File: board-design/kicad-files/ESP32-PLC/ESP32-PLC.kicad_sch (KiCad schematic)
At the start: 41 parts, among them J1 640456-3, J2 Conn_ARM_JTAG_SWD_10, J3 302-S101, J4 302-S101, Q1 BC817, Q2 BC817, U1 BD48ExxG, U2 ESP32-WROVER-E

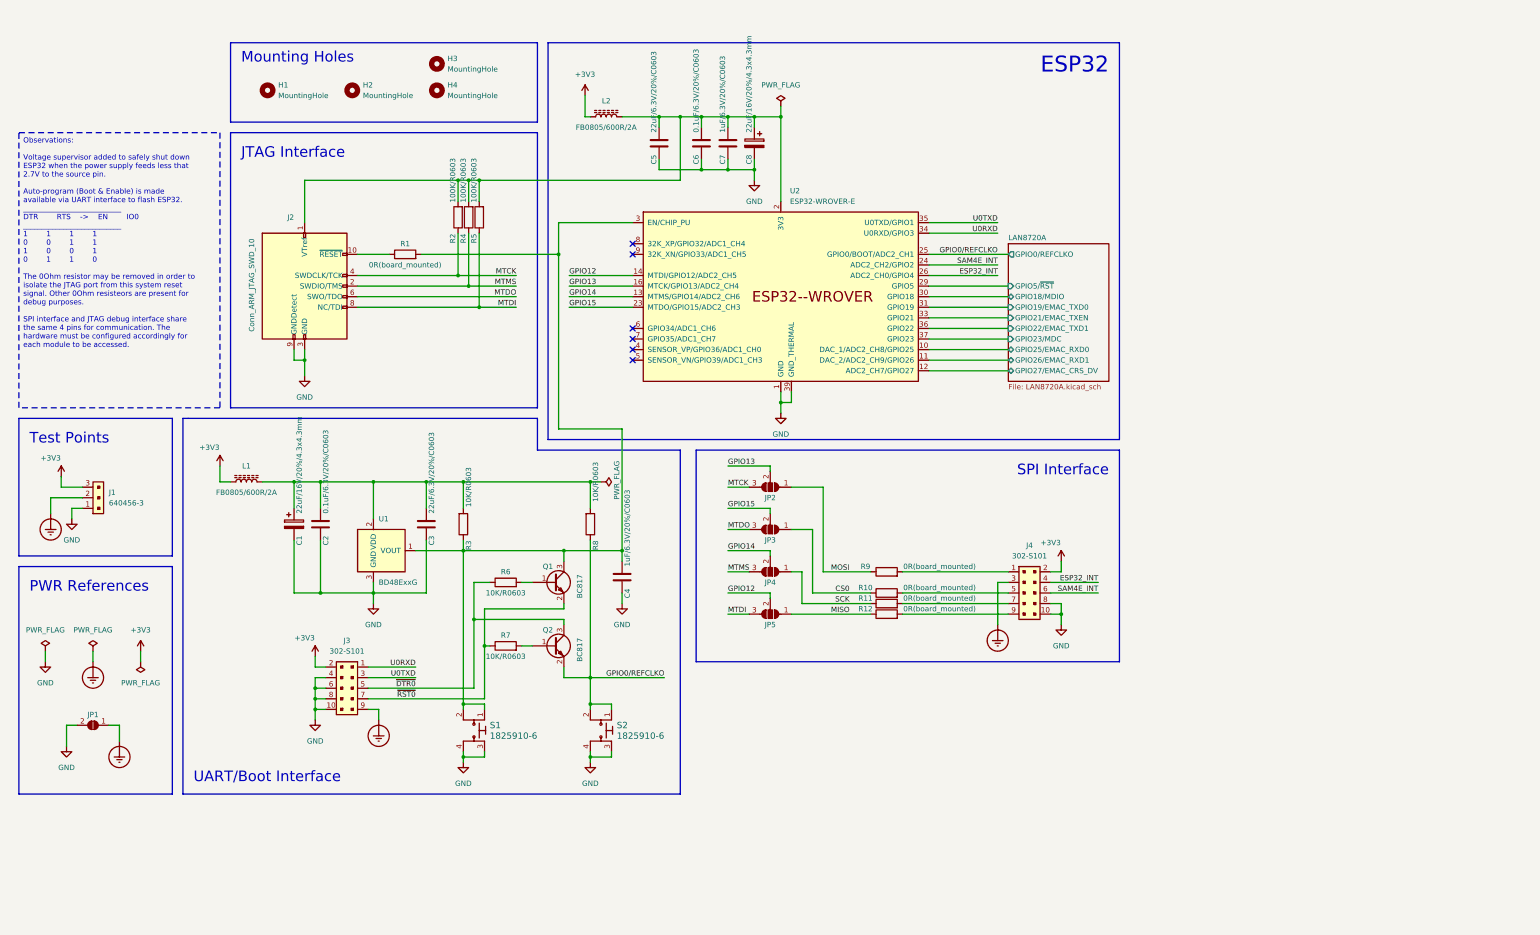
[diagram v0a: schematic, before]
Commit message: [UPDATE]
Work in progress.

Signed-off-by: Nicolae-Andrei Vasile <vasilenicolaeandrei@gmail.com>
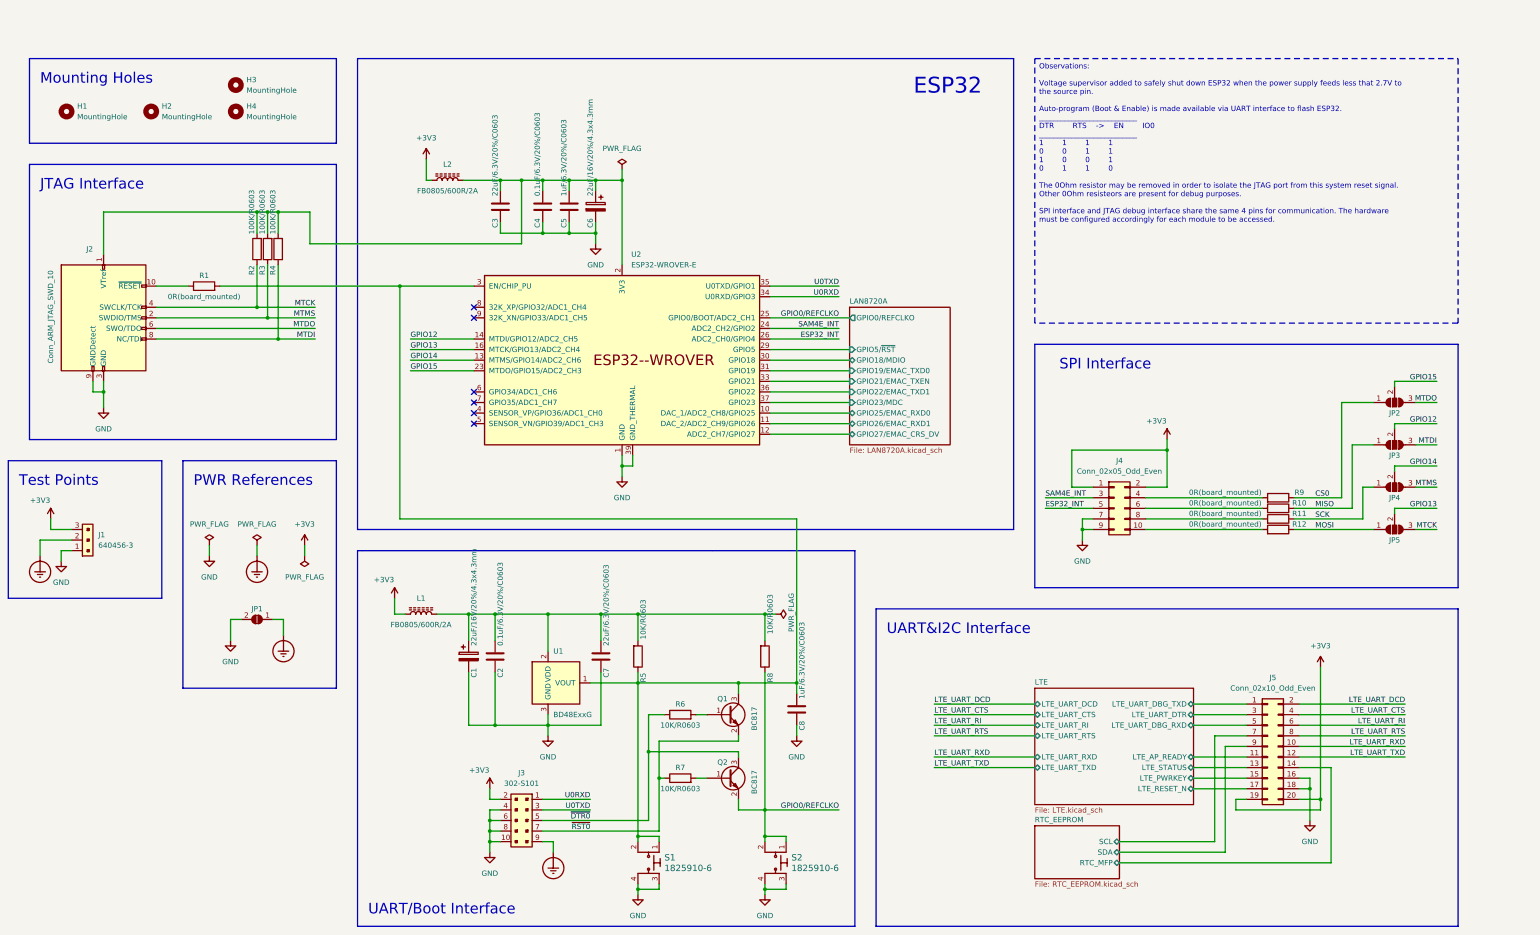
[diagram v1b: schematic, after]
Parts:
- removed J4: 302-S101, Connector_IDC:IDC-Header_2x05_P2.54mm_Vertical, symbol dk_Rectangular-Connectors-Headers-Male-Pins:302-S101
- added J4: Conn_02x05_Odd_Even, Connector_IDC:IDC-Header_2x05_P2.54mm_Vertical, symbol Connector_Generic:Conn_02x05_Odd_Even
- added J5: Conn_02x10_Odd_Even, Connector_IDC:IDC-Header_2x10_P2.54mm_Vertical, symbol Connector_Generic:Conn_02x10_Odd_Even
- renumbered C5 to C3, C6 to C4, C7 to C5, C8 to C6, C3 to C7, C4 to C8, JP3 to JP2, JP5 to JP3, JP2 to JP5, R4 to R3, R5 to R4, R3 to R5
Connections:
- net +3V3: now also J4.1 (Pin_1), J4.2 (Pin_2), J5.19 (Pin_19), J5.20 (Pin_20)
- net CS0: now also R9.1; no longer R10.1
- net ESP32_INT: now also J4.5 (Pin_5)
- net GND: now also J4.7 (Pin_7), J4.9 (Pin_9), J5.16 (Pin_16), J5.18 (Pin_18)
- net MISO: now also R10.1; no longer R12.1
- net MOSI: now also R12.1; no longer R9.1
- net SAM4E_INT: now also J4.3 (Pin_3)
- net at R9.2: now also J4.4 (Pin_4)
- net at R10.2: now also J4.6 (Pin_6)
- net at R11.2: now also J4.8 (Pin_8)
- net at R12.2: now also J4.10 (Pin_10)
- new net LTE/LTE_AP_READY: J5.11 (Pin_11)
- new net LTE/LTE_PWRKEY: J5.15 (Pin_15)
- new net LTE/LTE_RESET_N: J5.17 (Pin_17)
- new net LTE/LTE_STATUS: J5.13 (Pin_13)
- new net LTE/LTE_UART_DBG_RXD: J5.5 (Pin_5)
- new net LTE/LTE_UART_DBG_TXD: J5.1 (Pin_1)
- new net LTE/LTE_UART_DTR: J5.3 (Pin_3)
- new net LTE_UART_CTS: J5.4 (Pin_4)
- new net LTE_UART_DCD: J5.2 (Pin_2)
- new net LTE_UART_RI: J5.6 (Pin_6)
- new net LTE_UART_RTS: J5.8 (Pin_8)
- new net LTE_UART_RXD: J5.10 (Pin_10)
- new net LTE_UART_TXD: J5.12 (Pin_12)
- new net RTC_EEPROM/RTC_MFP: J5.14 (Pin_14)
- new net RTC_EEPROM/SCL: J5.7 (Pin_7)
- new net RTC_EEPROM/SDA: J5.9 (Pin_9)
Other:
- added sheet LTE (LTE.kicad_sch)
- added sheet RTC_EEPROM (RTC_EEPROM.kicad_sch)
- note added: "UART&I2C Interface"
- moved on the sheet: C1, C2, C3, C4, C5, C6, C7, C8, H1, H2, H3, H4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
